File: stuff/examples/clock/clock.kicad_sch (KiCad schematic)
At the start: 34 parts, among them SW1 SWITCH, SW2 SWITCH, U1 74LS393, U1 MAX7375AXR805, U10 4543, U11 4543, U12 4543, U13 4069, U14 4081, U15 HDSP-A153, U16 HDSP-A153, U17 HDSP-A153, U18 HDSP-A153, U19 HDSP-A153, U20 HDSP-A153, U4 4518, U5 4518, U6 4518, U7 4543, U8 4543, U9 4543

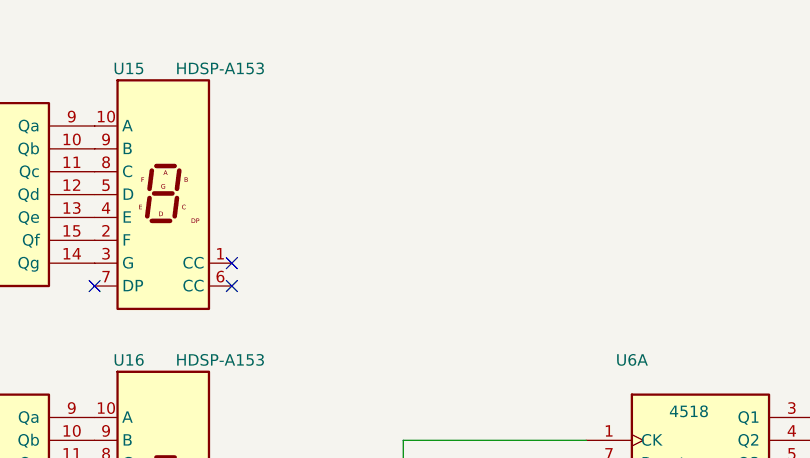
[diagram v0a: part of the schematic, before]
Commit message: cleanup
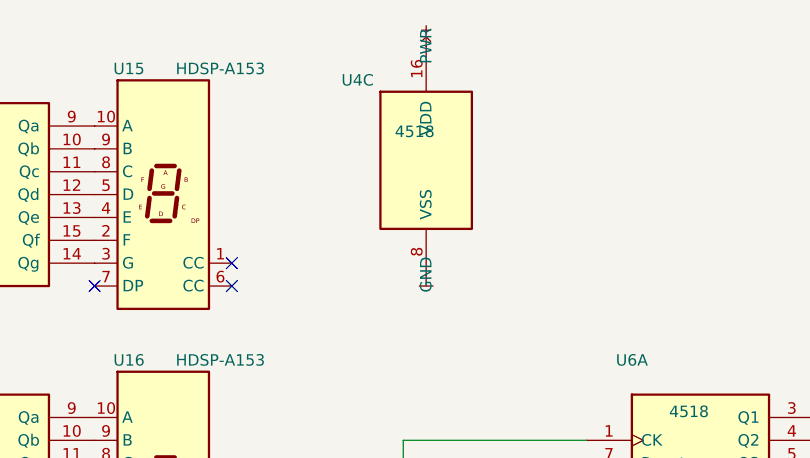
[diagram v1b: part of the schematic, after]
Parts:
- added unit 3 of U4
- U1: SymPartParam freq=16.384;start -> (none)
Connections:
- new net gnd: U4.8 (VSS)
- new net pwr: U4.16 (VDD)
